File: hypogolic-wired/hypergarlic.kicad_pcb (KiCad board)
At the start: 2 copper layers, 237.8 x 87.7 mm, 49 parts, among them J1 AudioJack4dpb, J2 AudioJack4dpb, SW10 SW_Push, SW11 SW_Push, SW11_r1 SW_Push, SW12 SW_Push, SW12_r1 SW_Push, SW13_r1 SW_Push, SW14 SW_Push, SW15 SW_Push, SW15_r1 SW_Push, SW16 SW_Push, SW16_r1 SW_Push, SW17 SW_Push, SW17_r1 SW_Push, SW18 SW_Push, SW18_r1 SW_Push, SW2 SW_Push, SW20 SW_Push, SW20_r1 SW_Push, SW21 SW_Push, SW21_r1 SW_Push, SW2_r1 SW_Push, SW3 SW_Push, SW3_r1 SW_Push, SW4 SW_Push, SW4_r1 SW_Push, SW5 SW_Push, SW5_r1 SW_Push, SW6 SW_Push, SW6_r1 SW_Push, SW7_r1 SW_Push, SW8 SW_Push, SW8_r1 SW_Push, SW9 SW_Push, SW9_r1 SW_Push, U1 ProMicro-kbd, U2 ProMicro-kbd

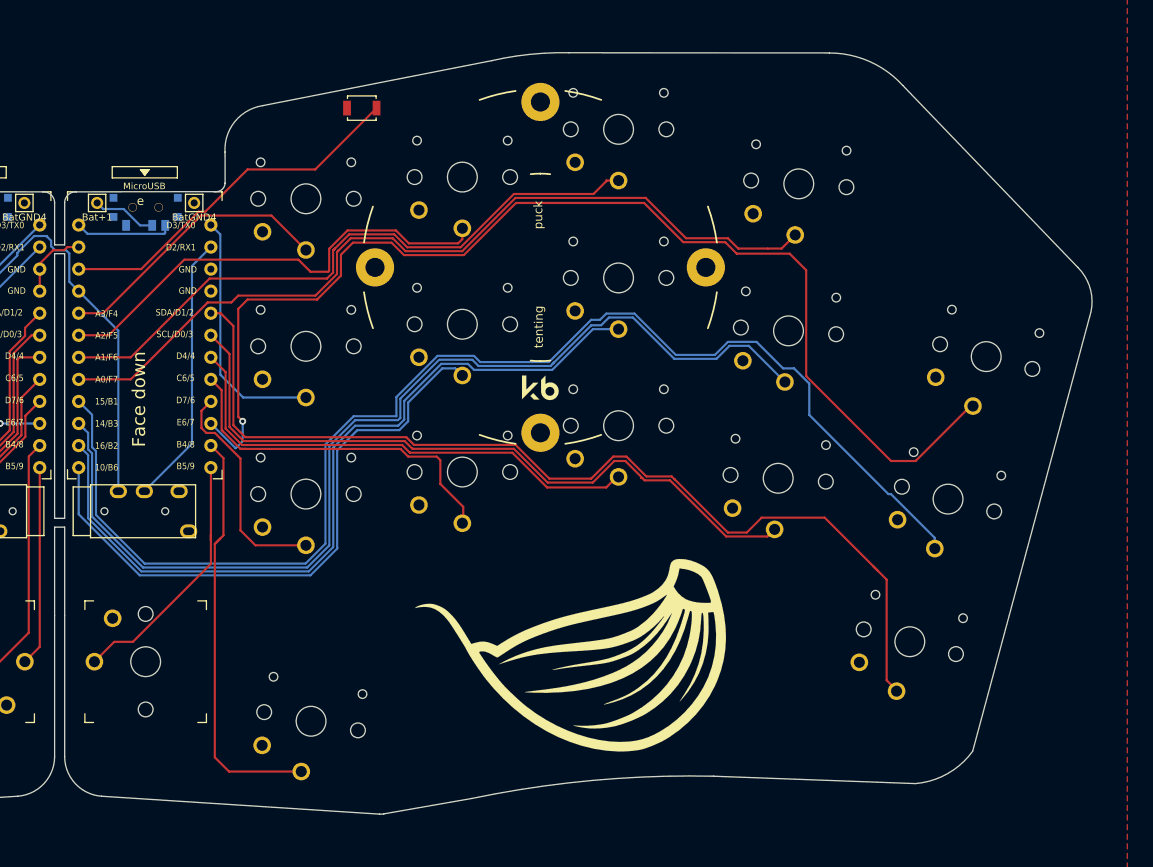
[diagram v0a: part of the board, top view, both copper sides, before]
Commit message: move apart a bit
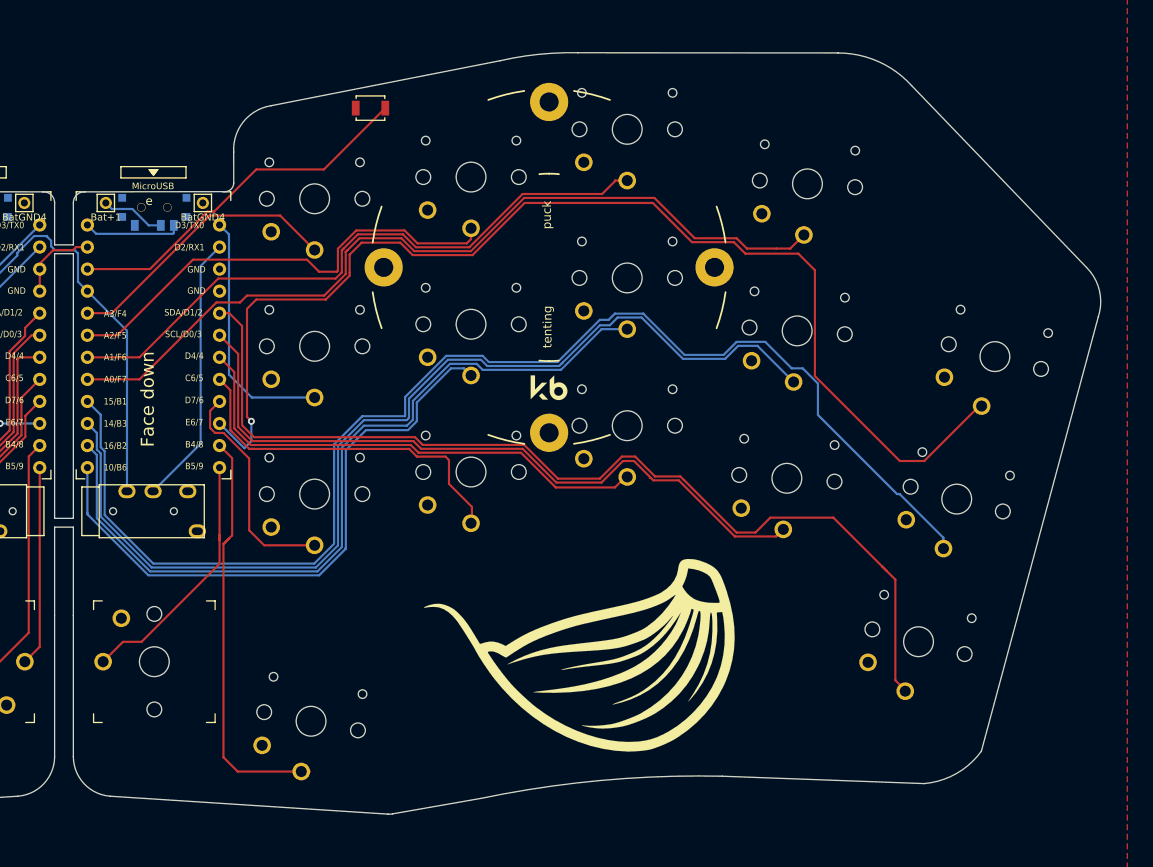
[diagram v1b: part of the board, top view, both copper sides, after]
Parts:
- moved Bat+1 1.00 mm to (139.4, 44.7)
- moved BatGND4 1.00 mm to (150.6, 44.7)
- moved G*** 1.00 mm to (195.8, 97.0)
- moved J1 1.00 mm to (138.7, 80.2)
- moved REF** 1.00 mm to (190.5, 52.1)
- moved RSW2 1.00 mm to (169.9, 33.8)
- moved SW11_r1 1.00 mm to (181.5, 58.7)
- moved SW12_r1 1.00 mm to (163.5, 61.2)
- moved SW13_r1 1.00 mm to (233.0, 95.2)
- moved SW15_r1 1.00 mm to (199.5, 70.4)
- moved SW16_r1 1.00 mm to (181.5, 75.7)
- moved SW17_r1 1.00 mm to (163.5, 78.2)
- moved SW18_r1 1.00 mm to (217.9, 76.4)
- moved SW20_r1 1.00 mm to (145.0, 97.5)
- moved SW2_r1 1.00 mm to (241.8, 62.4)
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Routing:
- net gnd: track 8.45 -> 9.45 mm
- net vcc: track 92.4 -> 93.4 mm
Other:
- board size 237.8 x 87.7 mm -> 238.8 x 87.7 mm
